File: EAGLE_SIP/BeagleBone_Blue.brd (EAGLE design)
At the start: 86.4 x 54.6 mm, 279 parts, among them M1 JST_ZH_2, M2 JST_ZH_2, M3 JST_ZH_2, M4 JST_ZH_2, P10 SCHA5B0200, Q3 MOSFET-N, U1 TPD4S012_DRY_6, U4 TPD4S012_DRY_6, U5 24LC_32AT-I/OT, U6 SN74LVC1G07_DCK_5, U7 TPS2051B_D_8, U8 MTFC4GLDEA, Y1 CM200C-32.768KAZF-UT, Y2 445C33D24M00000

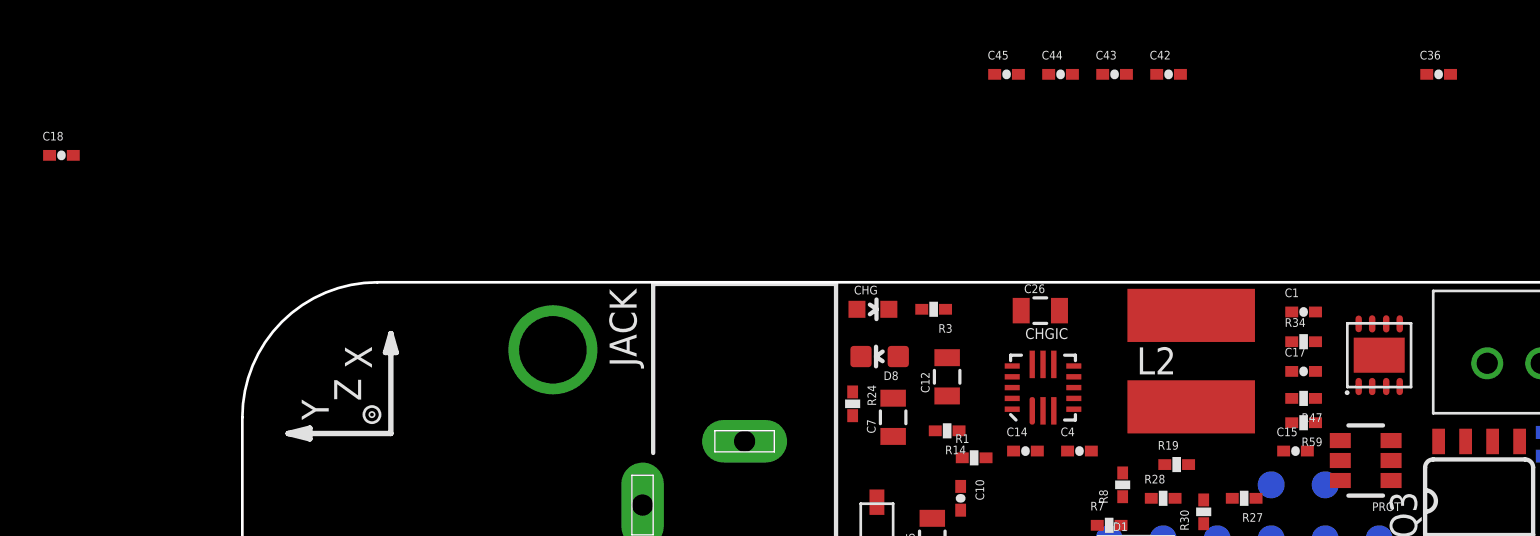
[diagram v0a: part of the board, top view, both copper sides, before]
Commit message: Rough place some parts
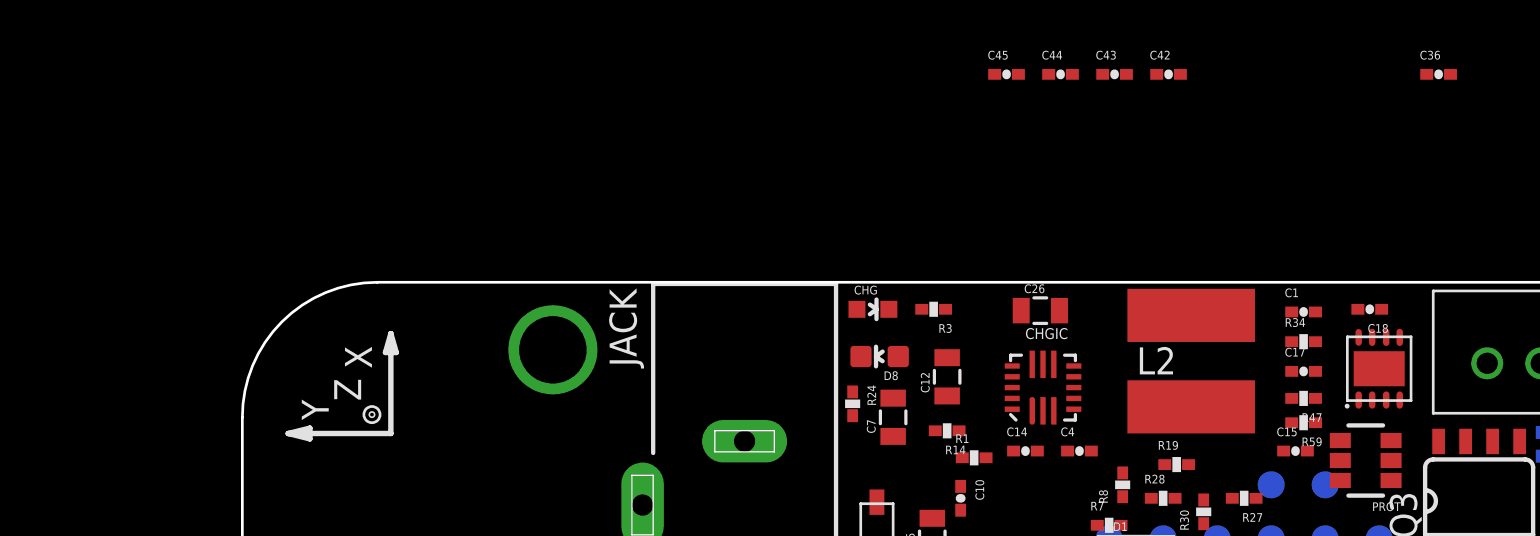
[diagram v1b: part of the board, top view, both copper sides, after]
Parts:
- moved C18 62.0 mm to (53.0, -1.27), turned to 180 degrees
- moved BAL 0.64 mm to (53.5, -4.06)
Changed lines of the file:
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@@
 <attribute name="NAME" x="58.801" y="-48.7045" size="1.016" layer="25" rot="R180"/>
 </element>
-<element name="BAL" library="Strawson_Eagle_Lib" package="8-SON_3X3MM" value="BQ29209" x="53.467" y="-3.429"/>
+<element name="BAL" library="Strawson_Eagle_Lib" package="8-SON_3X3MM" value="BQ29209" x="53.467" y="-4.064"/>
 <element name="BMP" library="SparkFun-Sensors" package="BMP180" value="BMP180" x="66.802" y="-29.845" rot="MR0"/>
 <element name="BOOT" library="SparkFun-Electromechanical" package="TACTILE-SWITCH-1101NE" value="SWITCH-MOMENTARY-2SMD-1101NE" x="4.699" y="-36.449" smashed="yes">
@@
 <element name="C16" library="SparkFun-Capacitors" package="0805" value="10uF 25V" x="24.765" y="-18.288"/>
 <element name="C17" library="Strawson_Eagle_Lib" package="0402-CAP" value="0.1uF" x="49.911" y="-4.191"/>
-<element name="C18" library="Strawson_Eagle_Lib" package="0402-CAP" value="0.1uF" x="-8.509" y="5.969"/>
+<element name="C18" library="Strawson_Eagle_Lib" package="0402-CAP" value="0.1uF" x="53.0225" y="-1.27" rot="R180"/>
 <element name="C19" library="Strawson_Eagle_Lib" package="0402-CAP" value="0.1uF" x="86.741" y="9.779"/>
 <element name="C2" library="Strawson_Eagle_Lib" package="0402-CAP" value="0.1uF" x="81.5975" y="-26.67"/>
@@
 <contactref element="R30" pad="2"/>
 <contactref element="BAL" pad="2"/>
-<wire x1="49.3522" y1="-4.191" x2="53.1368" y2="-4.9022" width="0" layer="19" extent="1-1"/>
+<wire x1="53.1368" y1="-5.5372" x2="52.4637" y2="-1.27" width="0" layer="19" extent="1-1"/>
+<wire x1="49.3522" y1="-4.191" x2="53.1368" y2="-5.5372" width="0" layer="19" extent="1-1"/>
 <wire x1="45.212" y1="-10.2362" x2="49.3522" y2="-4.191" width="0" layer="19" extent="1-1"/>
-<wire x1="-7.9502" y1="5.969" x2="45.212" y2="-10.2362" width="0" layer="19" extent="1-1"/>
 </signal>
 <signal name="BATT_MINUS">
@@
 <contactref element="PROT" pad="2"/>
 <wire x1="58.547" y1="-3.81" x2="87.2998" y2="9.779" width="0" layer="19" extent="1-1"/>
-<wire x1="54.4322" y1="-1.9558" x2="58.547" y2="-3.81" width="0" layer="19" extent="1-1"/>
-<wire x1="53.7972" y1="-1.9558" x2="54.4322" y2="-1.9558" width="0" layer="19" extent="1-1"/>
-<wire x1="50.4698" y1="-1.397" x2="53.7972" y2="-1.9558" width="0" layer="19" extent="1-1"/>
+<wire x1="54.4322" y1="-2.5908" x2="58.547" y2="-3.81" width="0" layer="19" extent="1-1"/>
+<wire x1="53.7972" y1="-2.5908" x2="54.4322" y2="-2.5908" width="0" layer="19" extent="1-1"/>
+<wire x1="53.5813" y1="-1.27" x2="53.7972" y2="-2.5908" width="0" layer="19" extent="1-1"/>
+<wire x1="50.4698" y1="-1.397" x2="53.5813" y2="-1.27" width="0" layer="19" extent="1-1"/>
 <wire x1="54.0258" y1="-8.382" x2="58.547" y2="-3.81" width="0" layer="19" extent="1-1"/>
 <wire x1="51.6382" y1="-9.3218" x2="54.0258" y2="-8.382" width="0" layer="19" extent="1-1"/>
+<wire x1="48.9712" y1="-7.9375" x2="51.6382" y2="-9.3218" width="0" layer="19" extent="1-1"/>
 <wire x1="56.261" y1="-13.087" x2="54.0258" y2="-8.382" width="0" layer="19" extent="1-1"/>
 <wire x1="57.531" y1="-13.087" x2="56.261" y2="-13.087" width="0" layer="19" extent="1-1"/>
 <wire x1="58.801" y1="-13.087" x2="57.531" y2="-13.087" width="0" layer="19" extent="1-1"/>
-<wire x1="48.9712" y1="-7.9375" x2="50.4698" y2="-1.397" width="0" layer="19" extent="1-1"/>
-<wire x1="-9.0678" y1="5.969" x2="48.9712" y2="-7.9375" width="0" layer="19" extent="1-1"/>
 </signal>
 <signal name="N$8">
@@
 <contactref element="C17" pad="2"/>
 <contactref element="BAL" pad="1"/>
-<wire x1="50.4698" y1="-4.191" x2="52.5018" y2="-4.9022" width="0" layer="19" extent="1-1"/>
+<wire x1="50.4698" y1="-4.191" x2="52.5018" y2="-5.5372" width="0" layer="19" extent="1-1"/>
 <wire x1="43.8658" y1="-10.16" x2="50.4698" y2="-4.191" width="0" layer="19" extent="1-1"/>
 </signal>
@@
 <contactref element="BAL" pad="7"/>
 <contactref element="C1" pad="1"/>
-<wire x1="50.4698" y1="-2.794" x2="53.1368" y2="-1.9558" width="0" layer="19" extent="1-1"/>
+<wire x1="50.4698" y1="-2.794" x2="53.1368" y2="-2.5908" width="0" layer="19" extent="1-1"/>
 <wire x1="49.3522" y1="-1.397" x2="50.4698" y2="-2.794" width="0" layer="19" extent="1-1"/>
 </signal>
@@
 <contactref element="BAL" pad="4"/>
 <contactref element="C19" pad="1"/>
-<wire x1="54.4322" y1="-4.9022" x2="86.1822" y2="9.779" width="0" layer="19" extent="1-1"/>
+<wire x1="54.4322" y1="-5.5372" x2="86.1822" y2="9.779" width="0" layer="19" extent="1-1"/>
 </signal>
 <signal name="N$50">
 <contactref element="R27" pad="2"/>
 <contactref element="BAL" pad="3"/>
-<wire x1="46.5582" y1="-10.16" x2="53.7972" y2="-4.9022" width="0" layer="19" extent="1-1"/>
+<wire x1="46.5582" y1="-10.16" x2="53.7972" y2="-5.5372" width="0" layer="19" extent="1-1"/>
 </signal>
 <signal name="CO">
 <contactref element="BAL" pad="8"/>
 <contactref element="R7" pad="1"/>
-<wire x1="40.2082" y1="-11.43" x2="52.5018" y2="-1.9558" width="0" layer="19" extent="1-1"/>
+<wire x1="40.2082" y1="-11.43" x2="52.5018" y2="-2.5908" width="0" layer="19" extent="1-1"/>
 </signal>
 <signal name="N$11">
